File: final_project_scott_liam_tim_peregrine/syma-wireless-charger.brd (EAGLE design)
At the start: 100 x 80 mm, 46 parts, among them U1 SAMD21E

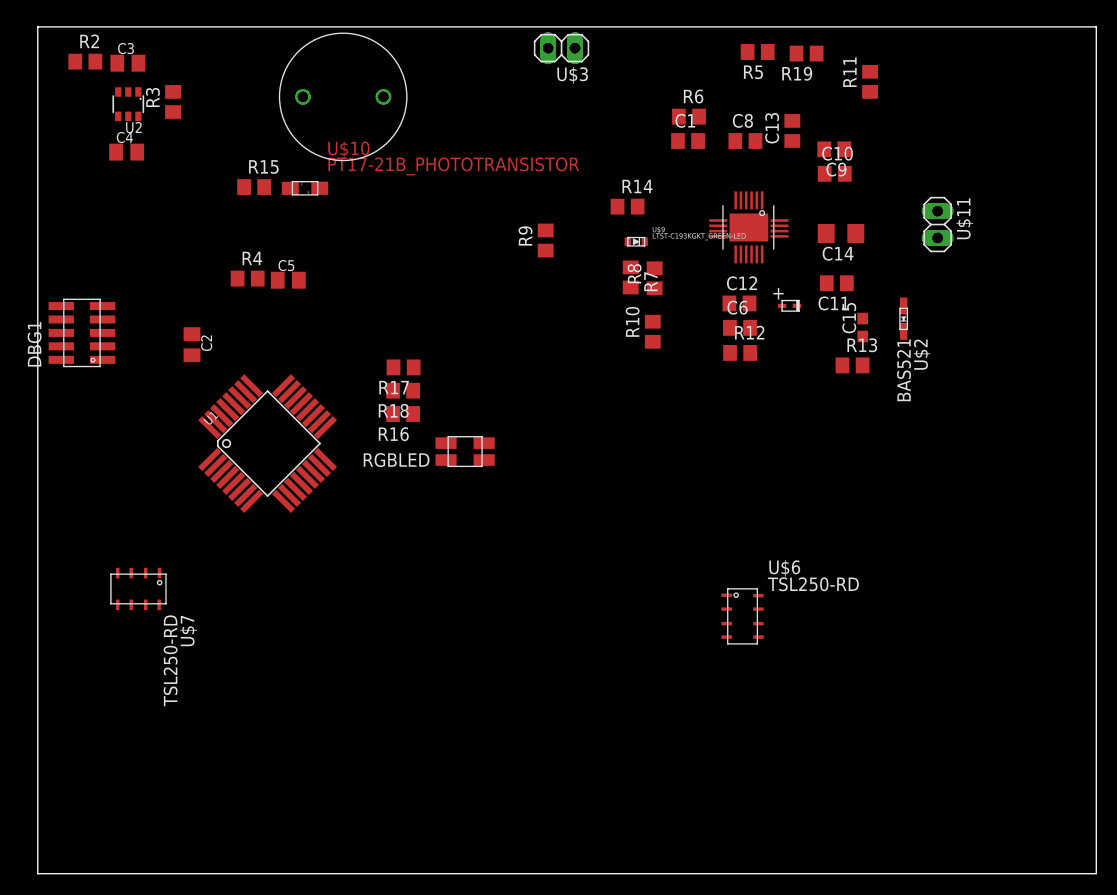
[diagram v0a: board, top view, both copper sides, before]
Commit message: mostly finished traces
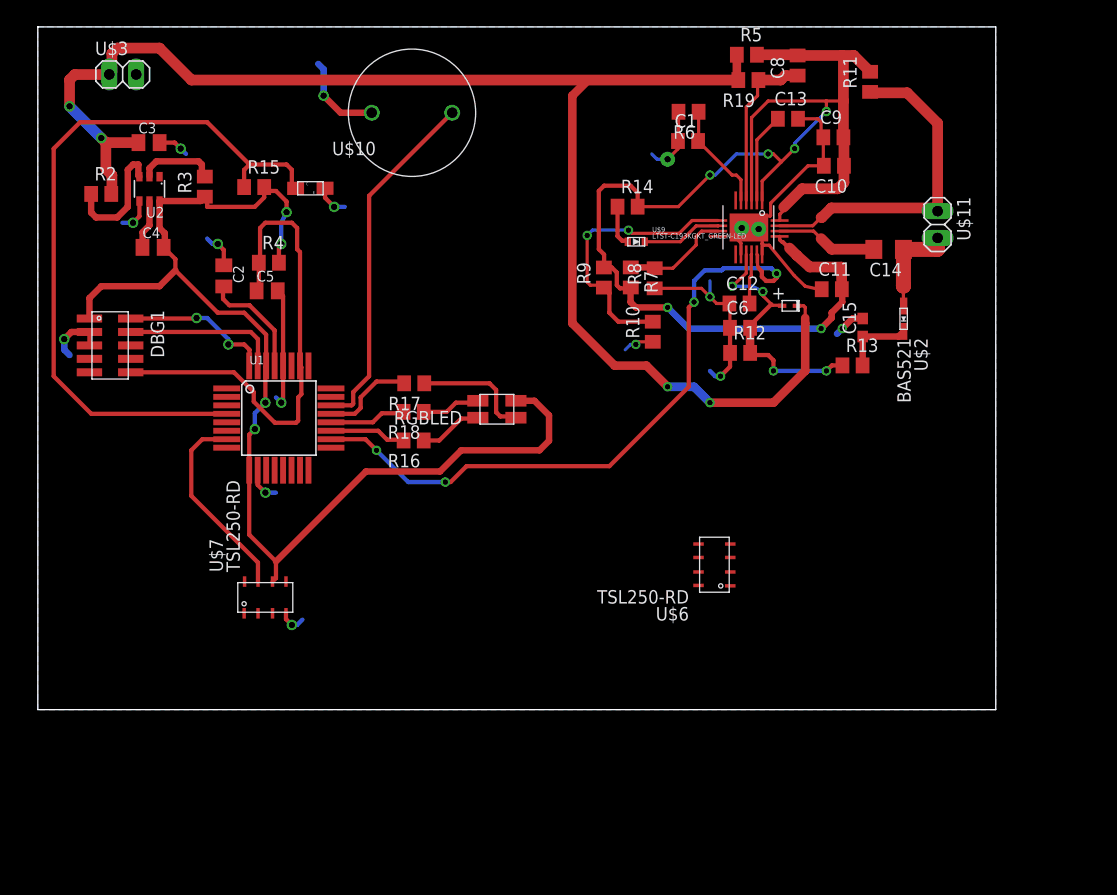
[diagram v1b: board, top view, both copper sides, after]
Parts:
- moved U$3 41.5 mm to (8.02, 75.5), turned to 0 degrees
- moved R2 12.6 mm to (5.99, 64.2)
- moved U$7 12.0 mm to (21.5, 26.1), turned to 90 degrees
- moved C4 9.34 mm to (10.9, 59.2)
- moved C8 8.67 mm to (71.8, 76.3), turned to 90 degrees
- moved R3 8.54 mm to (15.8, 64.9)
- moved U2 8.25 mm to (10.6, 64.7)
- moved C3 7.76 mm to (10.5, 69.1)
- moved DBG1 7.63 mm to (8.78, 52.5), turned to 270 degrees
- moved C2 7.16 mm to (17.6, 56.5)
- moved U$5 6.67 mm to (31.6, 71.9)
- moved R9 6.52 mm to (53.5, 56.3)
- moved R19 6.04 mm to (67.1, 75.0)
- moved U$6 5.56 mm to (63.9, 29.2), turned to 180 degrees
- moved U$4 5.00 mm to (45.2, 43.1)
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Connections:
- net GND: now also U$1.GND2
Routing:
- net +5V: track 0.00 -> 156.2 mm, vias 0 -> 4
- net N$20: track 0.00 -> 137.0 mm, vias 0 -> 6
- net VDD: track 0.00 -> 112.2 mm, vias 0 -> 4
- net GND: track 0.00 -> 106.9 mm, vias 0 -> 16
- net ALIGNED: track 0.00 -> 69.0 mm
- net PA17: track 0.00 -> 62.3 mm, vias 0 -> 4
- net RST: track 0.00 -> 46.9 mm
- net N$19: track 0.00 -> 33.5 mm
- net N$7: track 0.00 -> 31.7 mm
- net N$4: track 0.00 -> 26.4 mm, vias 0 -> 2
- net N$9: track 0.00 -> 24.9 mm, vias 0 -> 4
- net ENVSENSE: track 0.00 -> 18.8 mm
- net N$21: track 0.00 -> 15.7 mm
- net SWDCLK-PA30: track 0.00 -> 14.8 mm
- net SWDIO-PA31: track 0.00 -> 14.3 mm, vias 0 -> 2
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- added copper zone on layer 16, net GND
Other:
- board size 100 x 80 mm -> 90.5 x 64.5 mm
